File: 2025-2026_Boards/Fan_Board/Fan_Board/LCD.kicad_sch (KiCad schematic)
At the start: 1 part, among them J24 Conn_01x04_Pin

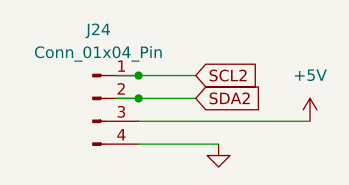
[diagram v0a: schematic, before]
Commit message: continued layout
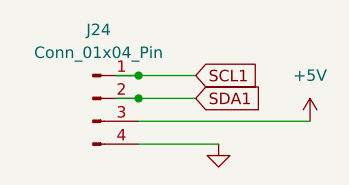
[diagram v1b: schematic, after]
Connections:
- net SCL2 renamed SCL1
- net SDA2 renamed SDA1
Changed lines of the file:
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@@
 		)
 	)
-	(global_label "SCL2"
+	(global_label "SCL1"
 		(shape input)
 		(at 134.62 74.93 0)
@@
 		)
 	)
-	(global_label "SDA2"
+	(global_label "SDA1"
 		(shape input)
 		(at 134.62 77.47 0)
